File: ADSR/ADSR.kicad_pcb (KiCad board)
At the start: 2 copper layers, 41 parts, among them J1 Panel, J2 Power, J3 Conn_01x04_Male, Q1 BC547, Q2 BC547, Q3 BC547, U1 LM358, U2 ICM7555

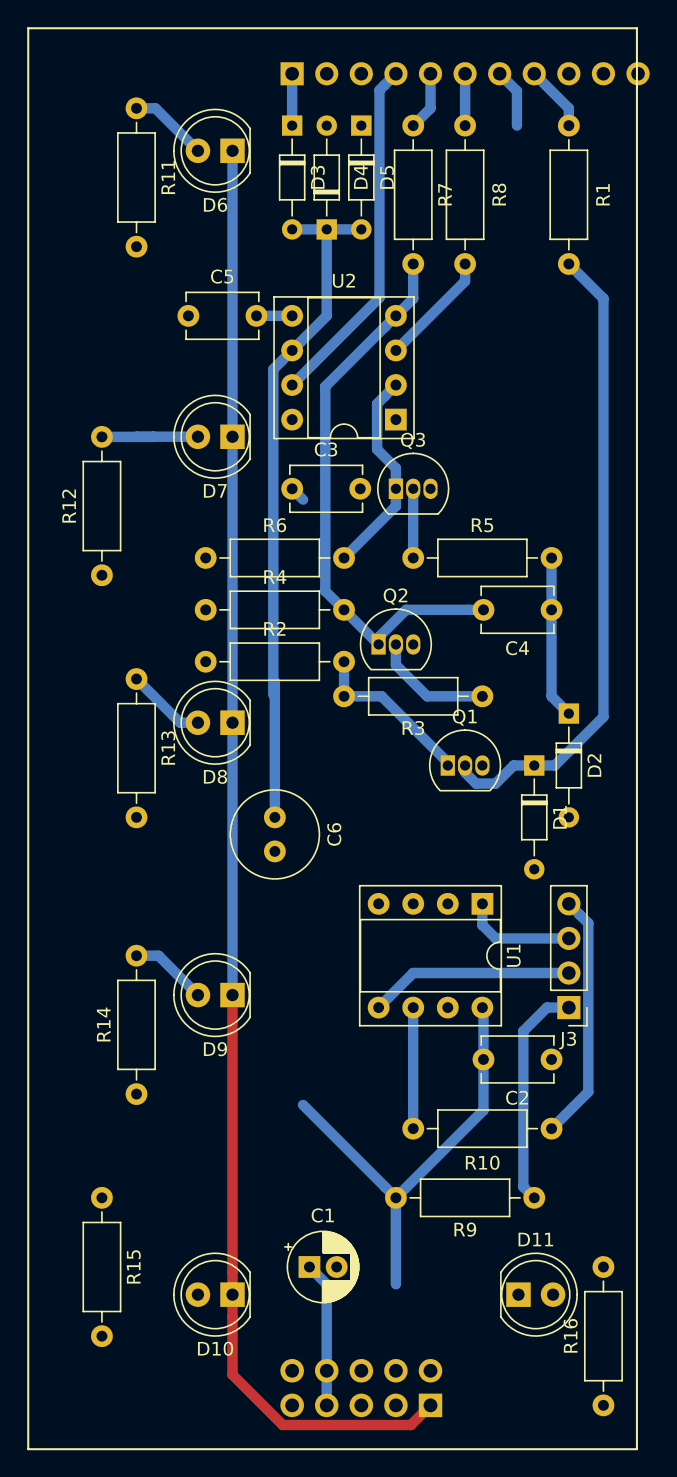
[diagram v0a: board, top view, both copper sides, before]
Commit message: update adsr pcb
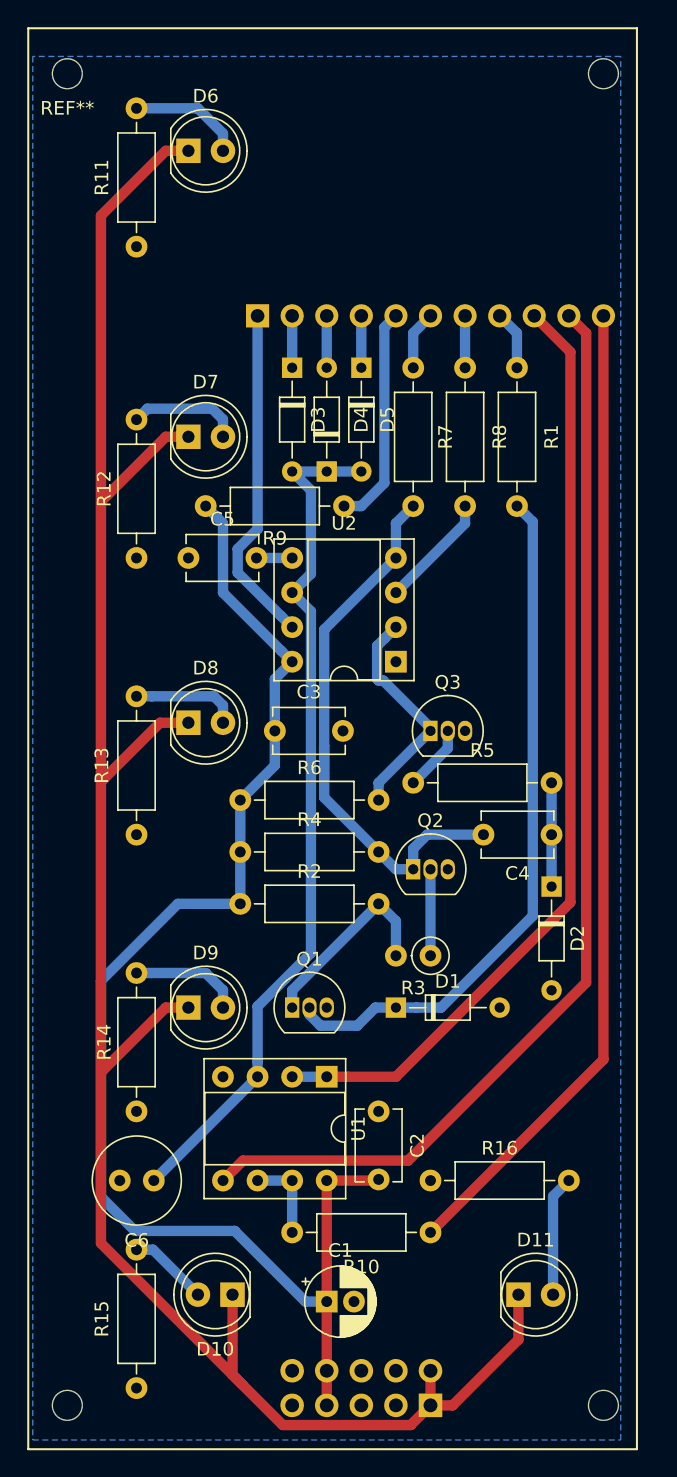
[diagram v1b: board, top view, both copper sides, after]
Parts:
- removed J3: Conn_01x04_Male, Connector_PinHeader_2.54mm:PinHeader_1x04_P2.54mm_Vertical
- added REF**: MountingHole_2.2mm_M2, MountingHole:MountingHole_2.2mm_M2, F.Cu at (142.2, 53.3)
- added REF**: MountingHole_2.2mm_M2, MountingHole:MountingHole_2.2mm_M2, F.Cu at (102.9, 53.3)
- added REF**: MountingHole_2.2mm_M2, MountingHole:MountingHole_2.2mm_M2, F.Cu at (142.2, 151.1)
- added REF**: MountingHole_2.2mm_M2, MountingHole:MountingHole_2.2mm_M2, F.Cu at (102.9, 151.1)
- R3: footprint Resistor_THT:R_Axial_DIN0207_L6.3mm_D2.5mm_P10.16mm_Horizontal -> Resistor_THT:R_Axial_DIN0207_L6.3mm_D2.5mm_P2.54mm_Vertical
- moved R9 52.7 mm to (123.2, 85.1)
- moved C6 28.1 mm to (109.2, 134.6), turned to 180 degrees
- moved Q1 21.1 mm to (119.4, 121.9)
- moved R16 20.8 mm to (129.5, 134.6), turned to 0 degrees
- moved D1 20.5 mm to (127.0, 121.9), turned to 0 degrees
- moved R3 19.4 mm to (129.5, 118.1)
- moved R1 18.2 mm to (135.9, 85.1)
- moved J1 18.0 mm to (116.8, 71.1)
- moved Q3 18.0 mm to (129.5, 101.6)
- moved R2 18.0 mm to (115.6, 114.3)
- moved R4 18.0 mm to (115.6, 110.5)
- moved R6 18.0 mm to (115.6, 106.7)
- moved C3 17.8 mm to (118.1, 101.6)
- moved D3 17.8 mm to (119.4, 74.9)
- moved D5 17.8 mm to (124.5, 74.9)
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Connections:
- J1 pad 1: Release_2 -> Sustain_3
- J1 pad 10: Net-(J1-Pad10) -> Sustain_2
- J1 pad 11: Net-(J1-Pad11) -> Decay_2
- J1 pad 2: Attack_2 -> Release_2
- J1 pad 3: Decay_1 -> Attack_2
- J1 pad 4: Sustain_3 -> Decay_1
- J1 pad 5: Release_1 -> Sustain_1
- J1 pad 6: Attack_1 -> Release_1
- J1 pad 7: IN -> Attack_1
- J1 pad 8: Net-(J1-Pad8) -> IN
- J1 pad 9: Net-(J1-Pad9) -> OUT
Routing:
- net Sustain_2: track 15.0 -> 82.2 mm
- net OUT: track 8.32 -> 69.9 mm
- net +15V: track 44.5 -> 102.1 mm
- net Decay_2: track 18.2 -> 72.6 mm
- net +5V: track 106.6 -> 160.3 mm
- net Net-(C6-Pad1): track 51.0 -> 63.6 mm
- net Net-(D11-Pad2): track 0.00 -> 8.86 mm
- net Net-(D10-Pad2): track 0.00 -> 5.88 mm
- net IN: track 9.20 -> 4.34 mm
- net Net-(C4-Pad1): track 12.0 -> 7.62 mm
- net Net-(D1-Pad1): track 47.4 -> 51.2 mm
- net Decay_1: track 0.00 -> 3.81 mm
- net Attack_2: track 0.00 -> 3.81 mm
- net Net-(D6-Pad2): track 5.80 -> 8.39 mm
- net Net-(R10-Pad1): track 8.89 -> 6.35 mm
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- added copper zone on B.Cu, net GND
